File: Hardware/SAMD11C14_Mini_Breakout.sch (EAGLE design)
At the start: 27 parts, among them J1 USB, U1 ATSAMD11C14, U2 3.3V

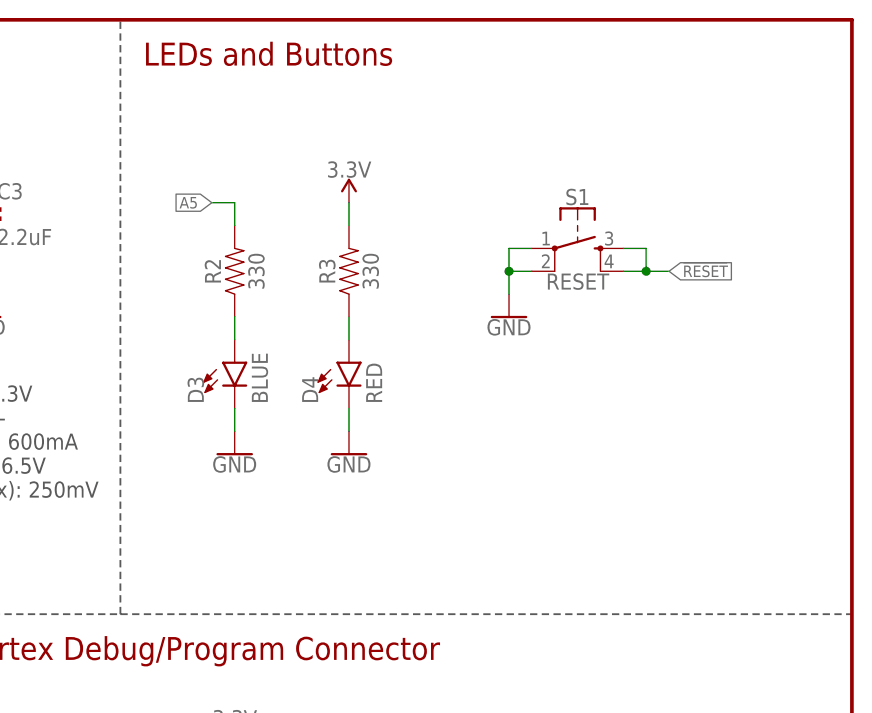
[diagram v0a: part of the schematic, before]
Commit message: Finished layout for v01
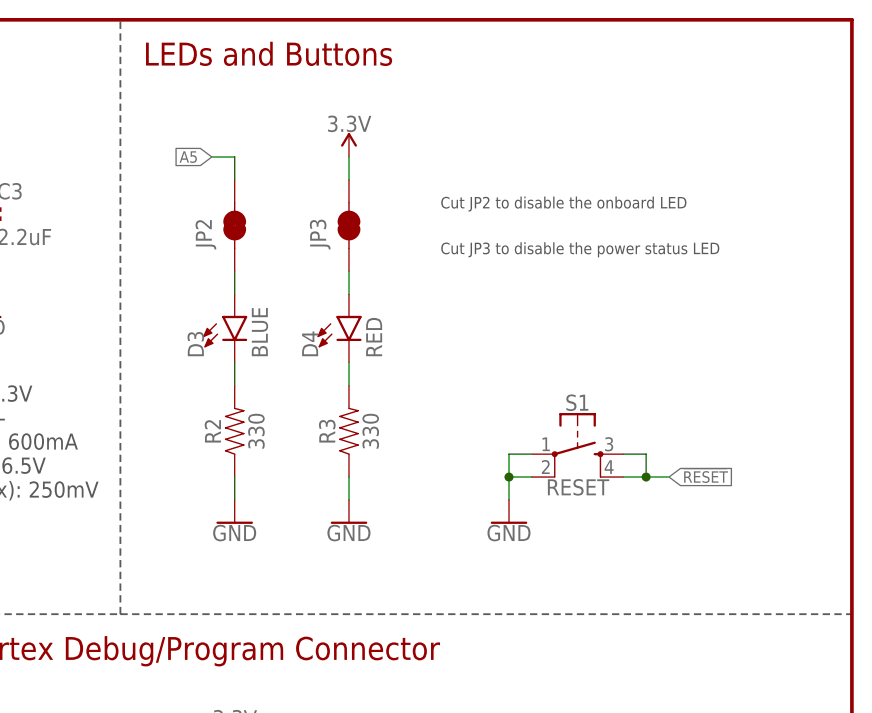
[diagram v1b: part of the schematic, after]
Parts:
- added JP2, JP3: JUMPER-SMT_2_NC_TRACE_NO-SILK, SparkFun-Jumpers:JUMPER-SMT_2_NC_TRACE_NO-SILK
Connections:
- new net N$3: D4.A, JP3.1
- new net N$5: D4.C, R3.2
- net 3.3V: now also JP3.2; no longer R3.2
- net A5: now also JP2.2; no longer R2.2
- net GND: now also R2.1, R3.1; no longer D3.C, D4.C
- net N$1: now also JP2.1; no longer R2.1
- net N$2: now also D3.C, R2.2; no longer D4.A, R3.1
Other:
- note added: "Cut JP2 to disable the onboard LED"
- note added: "Cut JP3 to disable the power status LED"
- moved on the sheet: D3, D4, R2, R3, S1
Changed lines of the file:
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@@
 <part name="SUPPLY8" library="SparkFun-PowerSymbols" deviceset="V_BATT" device=""/>
 <part name="SUPPLY13" library="SparkFun-PowerSymbols" deviceset="V_USB" device=""/>
+<part name="JP2" library="SparkFun-Jumpers" deviceset="JUMPER-SMT_2_NC_TRACE" device="_NO-SILK"/>
+<part name="JP3" library="SparkFun-Jumpers" deviceset="JUMPER-SMT_2_NC_TRACE" device="_NO-SILK"/>
 </parts>
 <sheets>
@@
 <text x="149.86" y="116.84" size="2.54" layer="94" align="top-left">Cortex Debug/Program Connector</text>
 <text x="149.86" y="76.2" size="2.54" layer="94" align="top-left">I/O pins</text>
+<text x="203.2" y="165.1" size="1.27" layer="97" align="center-left">Cut JP2 to disable the onboard LED</text>
+<text x="203.2" y="160.02" size="1.27" layer="97" align="center-left">Cut JP3 to disable the power status LED</text>
 </plain>
 <instances>
@@
 <instance part="GND5" gate="1" x="152.4" y="152.4"/>
 <instance part="SUPPLY6" gate="G$1" x="119.38" y="172.72"/>
-<instance part="R2" gate="G$1" x="180.34" y="157.48" rot="R90"/>
-<instance part="GND7" gate="1" x="180.34" y="137.16"/>
-<instance part="D3" gate="G$1" x="180.34" y="147.32"/>
+<instance part="R2" gate="G$1" x="180.34" y="139.7" rot="R90"/>
+<instance part="GND7" gate="1" x="180.34" y="129.54"/>
+<instance part="D3" gate="G$1" x="180.34" y="152.4"/>
 <instance part="JP1" gate="G$1" x="198.12" y="96.52"/>
 <instance part="SUPPLY9" gate="G$1" x="180.34" y="104.14"/>
 <instance part="GND8" gate="1" x="180.34" y="86.36"/>
-<instance part="S1" gate="G$1" x="218.44" y="160.02"/>
-<instance part="GND10" gate="1" x="210.82" y="152.4"/>
+<instance part="S1" gate="G$1" x="218.44" y="137.16"/>
+<instance part="GND10" gate="1" x="210.82" y="129.54"/>
 <instance part="R1" gate="G$1" x="33.02" y="91.44" rot="R90"/>
 <instance part="SUPPLY2" gate="G$1" x="33.02" y="99.06"/>
@@
 <instance part="H3" gate="G$1" x="238.76" y="33.02"/>
 <instance part="H4" gate="G$1" x="238.76" y="27.94"/>
-<instance part="R3" gate="G$1" x="193.04" y="157.48" rot="R90"/>
-<instance part="D4" gate="G$1" x="193.04" y="147.32"/>
-<instance part="GND9" gate="1" x="193.04" y="137.16"/>
-<instance part="SUPPLY11" gate="G$1" x="193.04" y="165.1"/>
+<instance part="R3" gate="G$1" x="193.04" y="139.7" rot="R90"/>
+<instance part="D4" gate="G$1" x="193.04" y="152.4"/>
+<instance part="GND9" gate="1" x="193.04" y="129.54"/>
+<instance part="SUPPLY11" gate="G$1" x="193.04" y="170.18"/>
 <instance part="D2" gate="G$1" x="88.9" y="170.18" smashed="yes" rot="R180">
 <attribute name="NAME" x="87.884" y="172.6946" size="1.778" layer="95"/>
@@
 <instance part="SUPPLY8" gate="G$1" x="175.26" y="63.5"/>
 <instance part="SUPPLY13" gate="G$1" x="195.58" y="63.5"/>
+<instance part="JP2" gate="G$1" x="180.34" y="162.56" smashed="yes" rot="R90">
+<attribute name="NAME" x="177.8" y="160.02" size="1.778" layer="95" font="vector" rot="R90"/>
+</instance>
+<instance part="JP3" gate="G$1" x="193.04" y="162.56" smashed="yes" rot="R90">
+<attribute name="NAME" x="190.5" y="160.02" size="1.778" layer="95" font="vector" rot="R90"/>
+</instance>
 </instances>
 <busses>
@@
 <segment>
 <pinref part="S1" gate="G$1" pin="2"/>
-<wire x1="213.36" y1="157.48" x2="210.82" y2="157.48" width="0.1524" layer="91"/>
+<wire x1="213.36" y1="134.62" x2="210.82" y2="134.62" width="0.1524" layer="91"/>
 <pinref part="GND10" gate="1" pin="GND"/>
-<wire x1="210.82" y1="157.48" x2="210.82" y2="154.94" width="0.1524" layer="91"/>
+<wire x1="210.82" y1="134.62" x2="210.82" y2="132.08" width="0.1524" layer="91"/>
 <pinref part="S1" gate="G$1" pin="1"/>
-<wire x1="213.36" y1="160.02" x2="210.82" y2="160.02" width="0.1524" layer="91"/>
-<wire x1="210.82" y1="160.02" x2="210.82" y2="157.48" width="0.1524" layer="91"/>
-<junction x="210.82" y="157.48"/>
+<wire x1="213.36" y1="137.16" x2="210.82" y2="137.16" width="0.1524" layer="91"/>
+<wire x1="210.82" y1="137.16" x2="210.82" y2="134.62" width="0.1524" layer="91"/>
+<junction x="210.82" y="134.62"/>
 </segment>
 <segment>
@@
 </segment>
 <segment>
-<pinref part="D3" gate="G$1" pin="C"/>
+<pinref part="R2" gate="G$1" pin="1"/>
 <pinref part="GND7" gate="1" pin="GND"/>
-<wire x1="180.34" y1="142.24" x2="180.34" y2="139.7" width="0.1524" layer="91"/>
-</segment>
-<segment>
-<pinref part="D4" gate="G$1" pin="C"/>
+<wire x1="180.34" y1="134.62" x2="180.34" y2="132.08" width="0.1524" layer="91"/>
+</segment>
+<segment>
+<pinref part="R3" gate="G$1" pin="1"/>
 <pinref part="GND9" gate="1" pin="GND"/>
-<wire x1="193.04" y1="142.24" x2="193.04" y2="139.7" width="0.1524" layer="91"/>
+<wire x1="193.04" y1="134.62" x2="193.04" y2="132.08" width="0.1524" layer="91"/>
 </segment>
 </net>
@@
 <segment>
 <pinref part="SUPPLY11" gate="G$1" pin="3.3V"/>
-<pinref part="R3" gate="G$1" pin="2"/>
-<wire x1="193.04" y1="165.1" x2="193.04" y2="162.56" width="0.1524" layer="91"/>
-</segment>
-</net>
-<net name="N$1" class="0">
-<segment>
-<pinref part="R2" gate="G$1" pin="1"/>
-<pinref part="D3" gate="G$1" pin="A"/>
-<wire x1="180.34" y1="152.4" x2="180.34" y2="149.86" width="0.1524" layer="91"/>
+<pinref part="JP3" gate="G$1" pin="2"/>
+<wire x1="193.04" y1="170.18" x2="193.04" y2="167.64" width="0.1524" layer="91"/>
 </segment>
 </net>
@@
 </segment>
 <segment>
-<pinref part="R2" gate="G$1" pin="2"/>
-<wire x1="180.34" y1="165.1" x2="180.34" y2="162.56" width="0.1524" layer="91"/>
-<wire x1="180.34" y1="165.1" x2="177.8" y2="165.1" width="0.1524" layer="91"/>
-<label x="177.8" y="165.1" size="1.27" layer="95" rot="R180" xref="yes"/>
+<wire x1="180.34" y1="170.18" x2="177.8" y2="170.18" width="0.1524" layer="91"/>
+<label x="177.8" y="170.18" size="1.27" layer="95" rot="R180" xref="yes"/>
+<pinref part="JP2" gate="G$1" pin="2"/>
+<wire x1="180.34" y1="170.18" x2="180.34" y2="167.64" width="0.1524" layer="91"/>
 </segment>
 </net>
@@
 </segment>
 <segment>
-<label x="228.6" y="157.48" size="1.27" layer="95" font="vector" xref="yes"/>
-<wire x1="226.06" y1="157.48" x2="228.6" y2="157.48" width="0.1524" layer="91"/>
+<label x="228.6" y="134.62" size="1.27" layer="95" font="vector" xref="yes"/>
+<wire x1="226.06" y1="134.62" x2="228.6" y2="134.62" width="0.1524" layer="91"/>
 <pinref part="S1" gate="G$1" pin="4"/>
-<wire x1="223.52" y1="157.48" x2="226.06" y2="157.48" width="0.1524" layer="91"/>
+<wire x1="223.52" y1="134.62" x2="226.06" y2="134.62" width="0.1524" layer="91"/>
 <pinref part="S1" gate="G$1" pin="3"/>
-<wire x1="223.52" y1="160.02" x2="226.06" y2="160.02" width="0.1524" layer="91"/>
-<wire x1="226.06" y1="160.02" x2="226.06" y2="157.48" width="0.1524" layer="91"/>
-<junction x="226.06" y="157.48"/>
+<wire x1="223.52" y1="137.16" x2="226.06" y2="137.16" width="0.1524" layer="91"/>
+<wire x1="226.06" y1="137.16" x2="226.06" y2="134.62" width="0.1524" layer="91"/>
+<junction x="226.06" y="134.62"/>
 </segment>
 <segment>
@@
 </segment>
 </net>
-<net name="N$2" class="0">
-<segment>
-<pinref part="R3" gate="G$1" pin="1"/>
-<pinref part="D4" gate="G$1" pin="A"/>
-<wire x1="193.04" y1="152.4" x2="193.04" y2="149.86" width="0.1524" layer="91"/>
-</segment>
-</net>
 <net name="V_BATT" class="0">
 <segment>
@@
 </segment>
 </net>
+<net name="N$1" class="0">
+<segment>
+<pinref part="JP2" gate="G$1" pin="1"/>
+<pinref part="D3" gate="G$1" pin="A"/>
+<wire x1="180.34" y1="157.48" x2="180.34" y2="154.94" width="0.1524" layer="91"/>
+</segment>
+</net>
+<net name="N$2" class="0">
+<segment>
+<pinref part="D3" gate="G$1" pin="C"/>
+<pinref part="R2" gate="G$1" pin="2"/>
+<wire x1="180.34" y1="147.32" x2="180.34" y2="144.78" width="0.1524" layer="91"/>
+</segment>
+</net>
+<net name="N$3" class="0">
+<segment>
+<pinref part="JP3" gate="G$1" pin="1"/>
+<pinref part="D4" gate="G$1" pin="A"/>
+<wire x1="193.04" y1="157.48" x2="193.04" y2="154.94" width="0.1524" layer="91"/>
+</segment>
+</net>
+<net name="N$5" class="0">
+<segment>
+<pinref part="D4" gate="G$1" pin="C"/>
+<pinref part="R3" gate="G$1" pin="2"/>
+<wire x1="193.04" y1="147.32" x2="193.04" y2="144.78" width="0.1524" layer="91"/>
+</segment>
+</net>
